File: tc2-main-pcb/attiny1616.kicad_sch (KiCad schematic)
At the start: 20 parts, among them J104 Conn_02x03_Odd_Even, U117 ATtiny1616-M

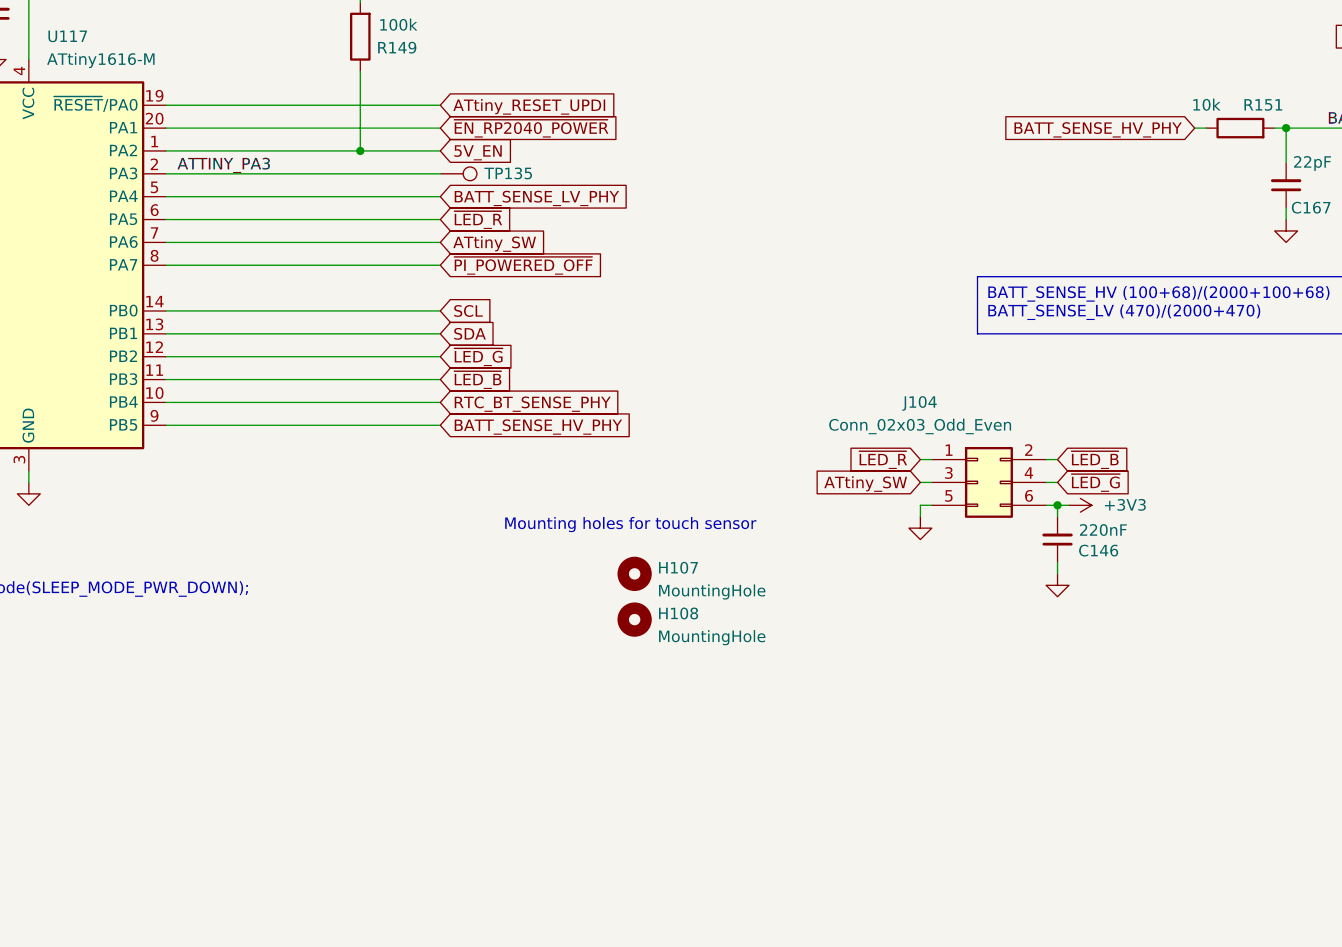
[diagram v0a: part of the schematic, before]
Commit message: Tidy up
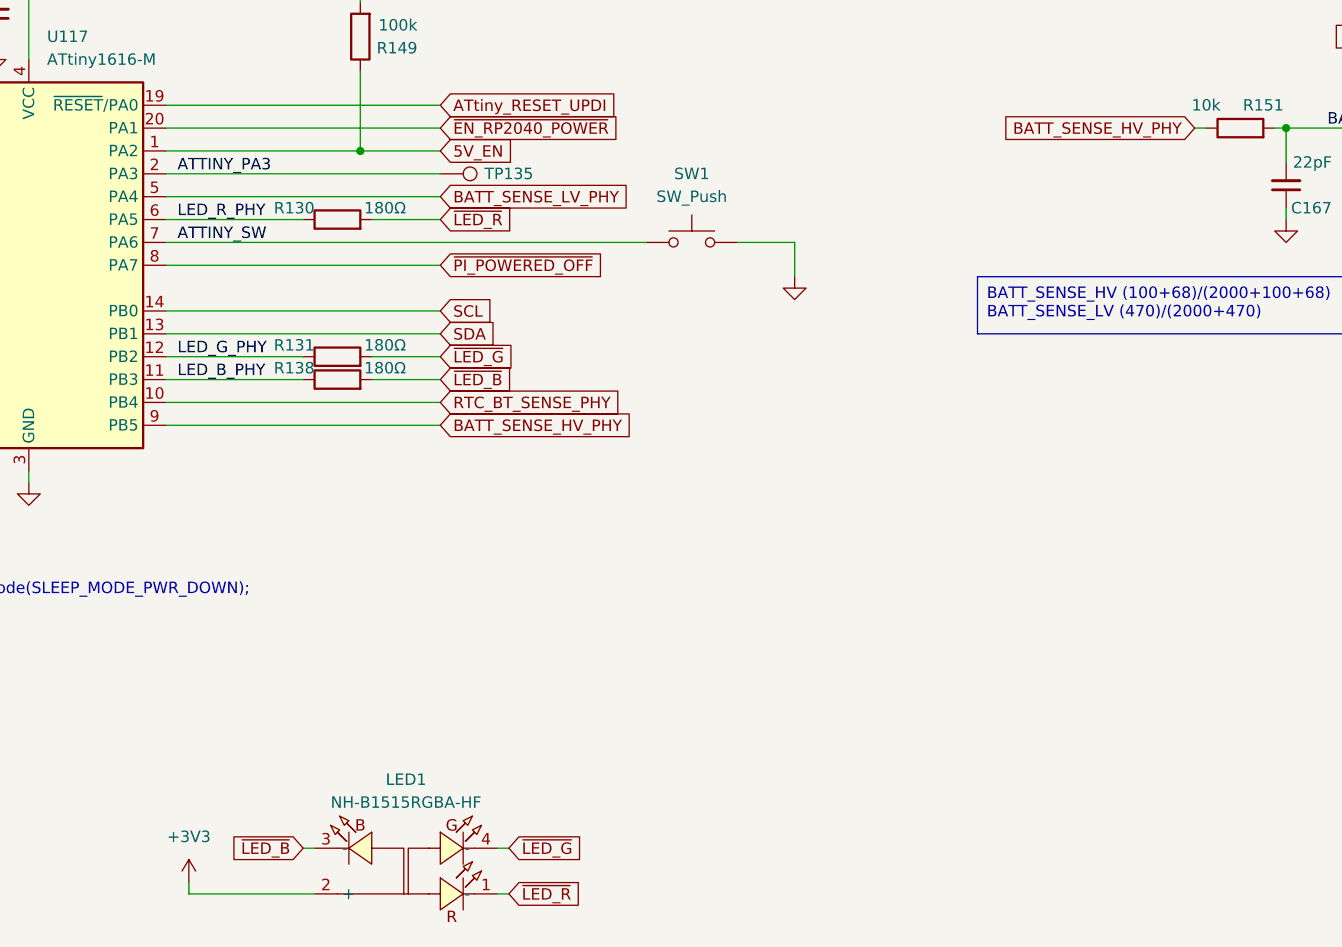
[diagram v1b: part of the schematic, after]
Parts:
- removed C146: 220nF, Capacitor_SMD:C_0402_1005Metric, symbol Device:C_Small
- removed H107, H108: MountingHole, cacophony-library:MountingHole_2.2mm_M2, symbol Mechanical:MountingHole
- removed J104: Conn_02x03_Odd_Even, cacophony-library:mic-pcb, symbol Connector_Generic:Conn_02x03_Odd_Even
- added LED1: NH-B1515RGBA-HF, cacophony-library:LED-ARRAY-SMD_4P-L1.6-W1.5-TL_NH-B1515RGBA, symbol cacophony-library:NH-B1515RGBA-HF
- added R130, R131, R138: 180Ω, Resistor_SMD:R_0402_1005Metric, symbol Device:R
- added SW1: SW_Push, cacophony-library:SW_PUSH_6mm_11mmh, symbol Switch:SW_Push
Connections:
- net +3V3: now also LED1.2 (+)
- net GND: now also SW1.2
- net ~{LED_B}: now also LED1.3 (-), R138.2; no longer U117.11 (PB3)
- net ~{LED_G}: now also LED1.4 (-), R131.2; no longer U117.12 (PB2)
- net ~{LED_R}: now also LED1.1 (-), R130.2; no longer U117.6 (PA5)
- net ATtiny_SW renamed ATTINY_SW
- net ATTINY_SW: now also SW1.1
- new net LED_B_PHY: R138.1, U117.11 (PB3)
- new net LED_G_PHY: R131.1, U117.12 (PB2)
- new net LED_R_PHY: R130.1, U117.6 (PA5)
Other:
- note removed: "Mounting holes for touch sensor"
